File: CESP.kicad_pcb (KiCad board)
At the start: 2 copper layers, 17 parts, among them K1 CONN_3, U1 7555, U2 LM741, U3 7805-REG

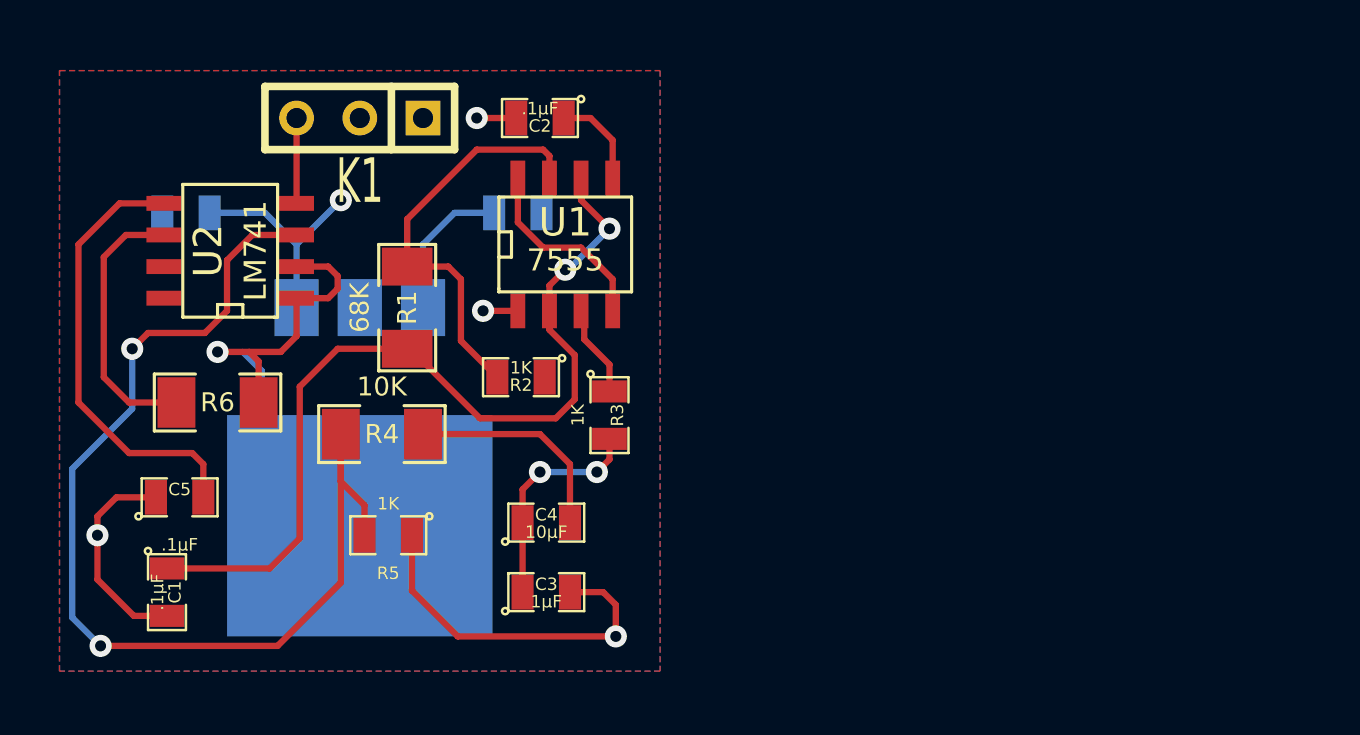
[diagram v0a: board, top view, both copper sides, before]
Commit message: Several PCB layout drafts later...
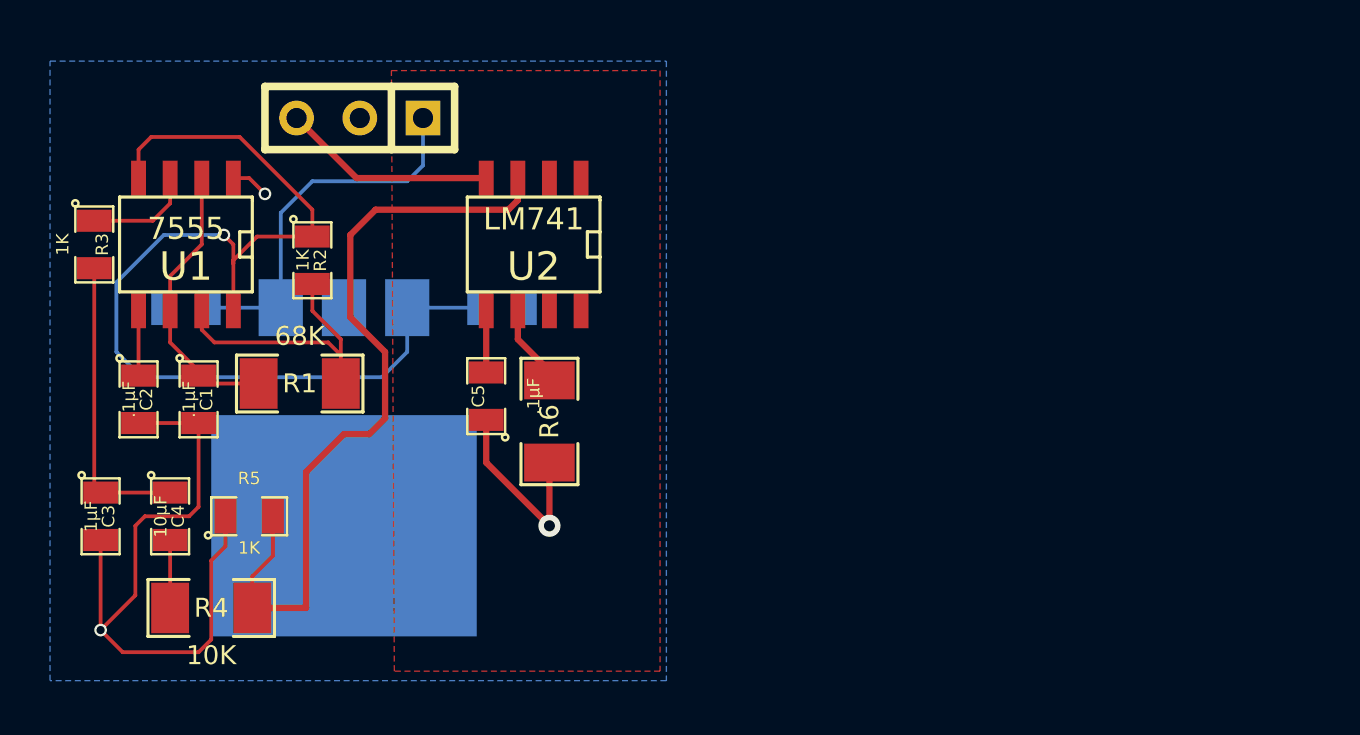
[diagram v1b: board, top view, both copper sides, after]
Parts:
- moved R3 21.8 mm to (189.4, 135.9)
- moved C2 19.7 mm to (191.1, 142.1), turned to 270 degrees
- moved C3 18.2 mm to (189.6, 146.8), turned to 270 degrees
- moved U1 15.2 mm to (193.0, 135.9), turned to 180 degrees
- moved C4 15.1 mm to (192.4, 146.8), turned to 270 degrees
- moved R6 13.4 mm to (207.6, 143.0), turned to 90 degrees
- moved C5 13.0 mm to (205.1, 142.0), turned to 90 degrees
- moved U2 12.2 mm to (207.0, 135.9), turned to 180 degrees
- moved R4 9.79 mm to (194.1, 150.5), turned to 180 degrees
- moved R2 9.61 mm to (198.1, 136.5), turned to 270 degrees
- moved C1 7.85 mm to (193.5, 142.1)
- moved R5 5.64 mm to (195.6, 146.8), turned to 0 degrees
- moved R1 5.29 mm to (197.6, 141.5), turned to 180 degrees
- moved C7 3.86 mm to (205.7, 138.4)
- moved C6 3.81 mm to (193.0, 138.4)
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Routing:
- net N-0000010: track 13.7 -> 42.6 mm, vias 0 -> 1
- net N-000008: track 35.9 -> 11.5 mm, vias 2 -> 0
- net N-000007: track 17.8 -> 2.48 mm
- net N-000005: track 44.2 -> 31.9 mm, vias 2 -> 0
- net N-000006: track 10.9 -> 3.32 mm
- net N-0000013: track 8.75 -> 2.73 mm
- net VCC: track 9.07 -> 15.1 mm, vias 1 -> 0
- net N-0000011: track 16.7 -> 11.2 mm
- net -9V: track 3.43 -> 8.62 mm
- net N-0000014: track 8.95 -> 11.9 mm, vias 2 -> 0
- net (no net): track 2.35 -> 0.00 mm
- net N-0000012: track 3.86 -> 2.60 mm
- net GND: track 37.4 -> 36.6 mm, vias 5 -> 3
- net N-000009: track 3.71 -> 4.35 mm
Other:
- rule trace_min: 0.254 -> 0.1524
- rule via_min_drill: 0.508 -> 0.3302
- rule via_min_size: 0.889 -> 0.508

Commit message: And yet further PCB layout drafts...
... I'm beginning to truly despise this board.  I think it has it out
for me.
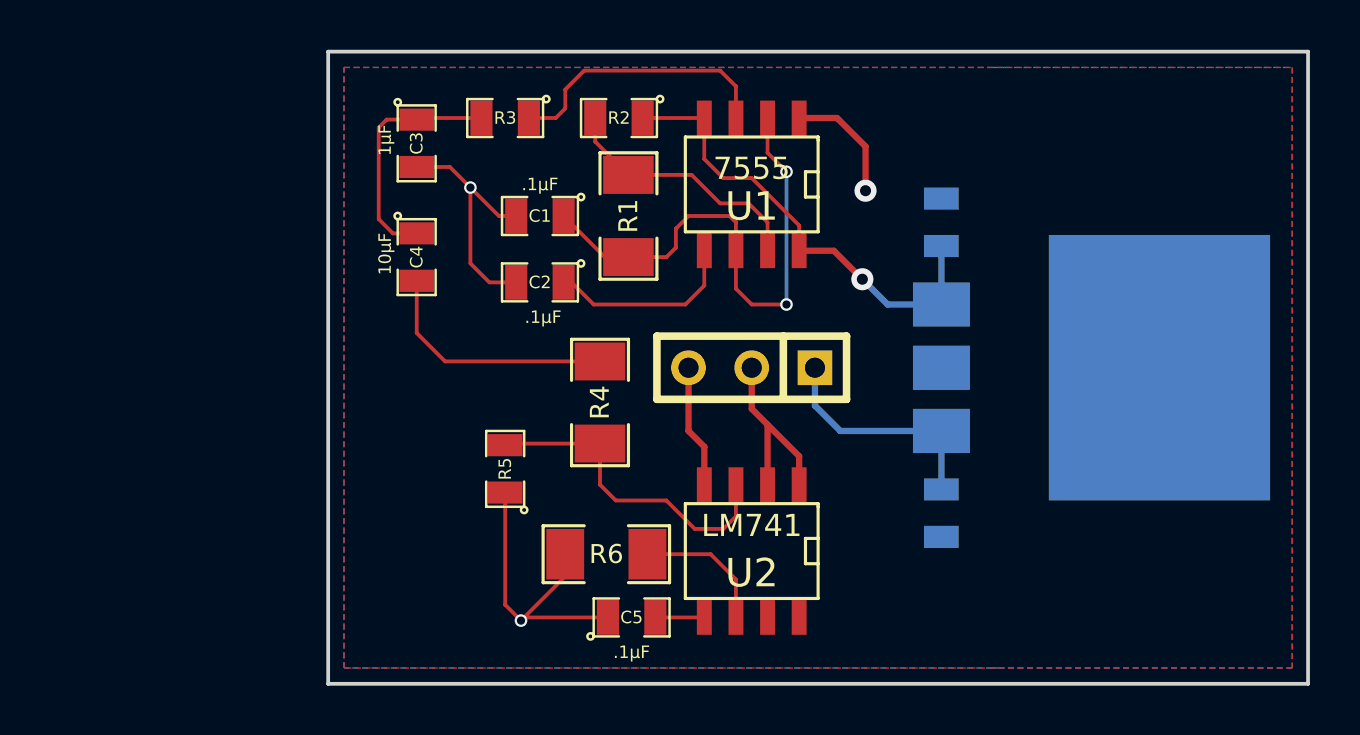
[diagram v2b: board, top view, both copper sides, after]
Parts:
- moved C6 31.5 mm to (223.4, 146.7), turned to 270 degrees
- moved U3 24.1 mm to (223.4, 140.8), turned to 90 degrees
- moved U1 22.9 mm to (215.8, 133.5)
- moved C3 19.6 mm to (202.3, 131.8)
- moved K1 18.7 mm to (215.8, 140.8)
- moved C7 18.0 mm to (223.4, 135.0), turned to 90 degrees
- moved R4 17.7 mm to (209.7, 142.2), turned to 90 degrees
- moved R3 17.3 mm to (205.9, 130.8), turned to 180 degrees
- moved C2 16.8 mm to (207.3, 137.4), turned to 180 degrees
- moved C1 15.6 mm to (207.3, 134.7), turned to 180 degrees
- moved U2 15.1 mm to (215.8, 148.2)
- moved R1 14.8 mm to (210.8, 134.7), turned to 270 degrees
- moved C4 14.4 mm to (202.3, 136.4)
- moved R2 13.6 mm to (210.4, 130.8), turned to 180 degrees
- moved C5 10.6 mm to (210.9, 150.9), turned to 0 degrees
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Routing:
- net N-0000010: track 42.6 -> 19.0 mm
- net N-000005: track 31.9 -> 13.2 mm
- net N-000008: track 11.5 -> 21.6 mm, vias 0 -> 2
- net N-0000013: track 2.73 -> 9.93 mm
- net N-000009: track 4.35 -> 11.1 mm
- net VCC: track 15.1 -> 9.37 mm
- net N-0000012: track 2.60 -> 7.73 mm
- net -9V: track 8.62 -> 4.96 mm
- net N-0000014: track 11.9 -> 9.73 mm
- net N-000006: track 3.32 -> 5.50 mm
- net GND: track 36.6 -> 35.2 mm
- net N-0000011: track 11.2 -> 10.4 mm
- net N-000007: track 2.48 -> 1.97 mm
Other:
- board outline added: 39.4 x 25.4 mm
